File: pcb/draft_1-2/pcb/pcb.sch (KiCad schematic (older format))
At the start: 35 parts, among them J1 USB4110-GF-A, J2 SWD, U1 H3LIS200DLTR, U2 ATSAML21J16B-AUT, U3 BQ25155

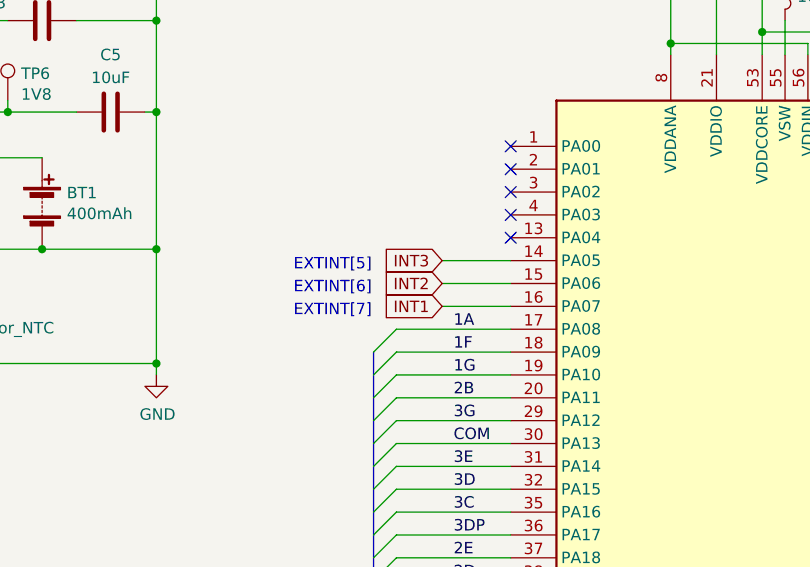
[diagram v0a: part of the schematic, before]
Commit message: v1.2 draft
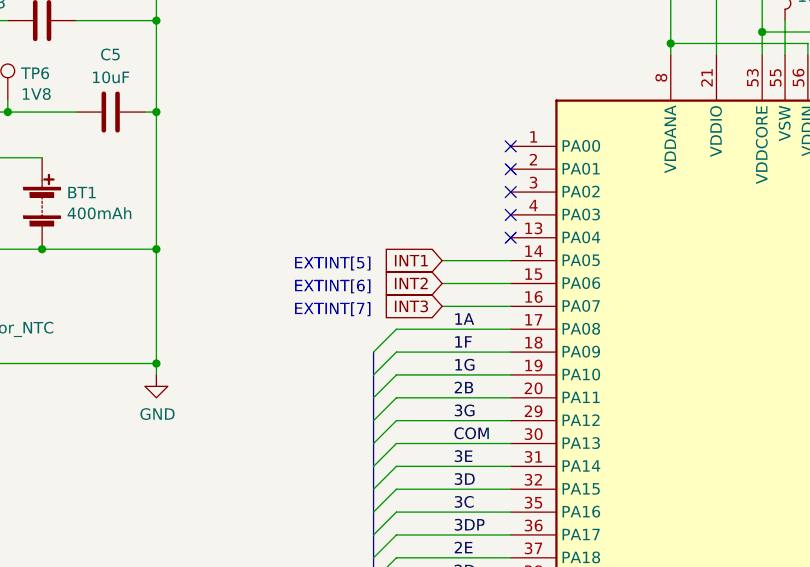
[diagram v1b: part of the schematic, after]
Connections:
- net INT1: now also U2.14 (PA05); no longer U2.16 (PA07)
- net INT3: now also U2.16 (PA07); no longer U2.14 (PA05)
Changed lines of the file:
@@
 Wire Wire Line
 	8900 2000 9450 2000
-Text GLabel 7500 3200 0    50   Input ~ 0
+Text GLabel 7500 3000 0    50   Input ~ 0
 INT1
 Text GLabel 7500 3100 0    50   Input ~ 0
 INT2
-Text GLabel 7500 3000 0    50   Input ~ 0
+Text GLabel 7500 3200 0    50   Input ~ 0
 INT3
 Text GLabel 10050 5300 3    50   Input ~ 0
